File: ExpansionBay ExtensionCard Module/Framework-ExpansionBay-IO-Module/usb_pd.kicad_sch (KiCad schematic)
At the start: 9 parts, among them U2 CYPD4126-40LQXIT

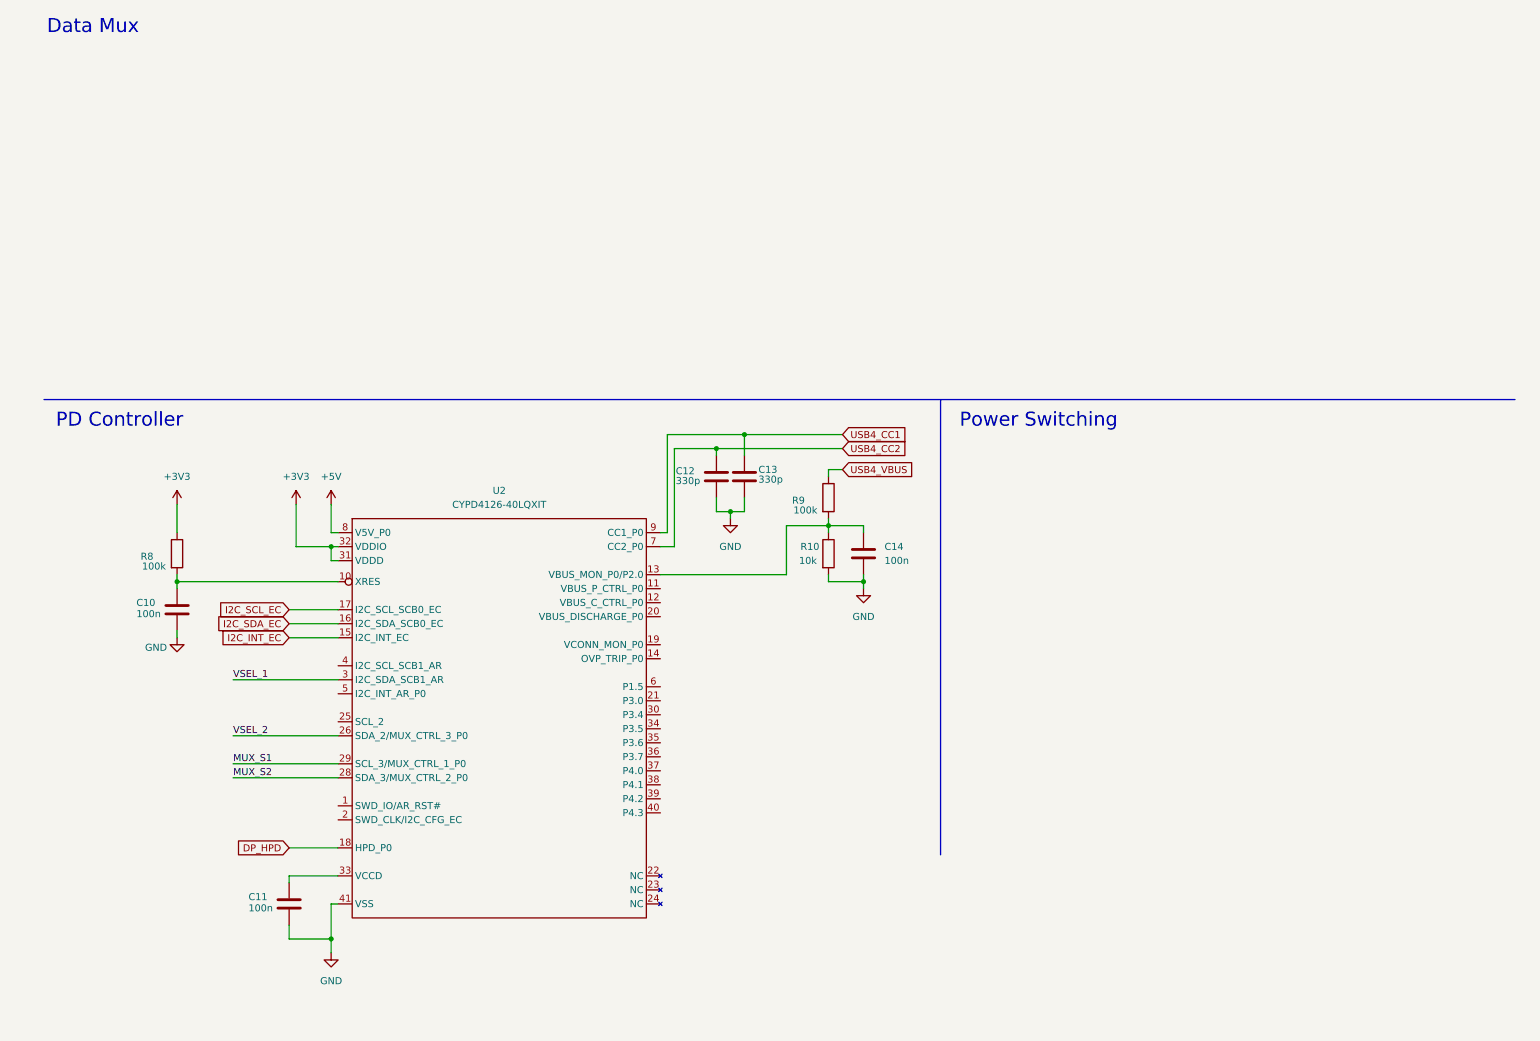
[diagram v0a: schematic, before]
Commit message: partial redesign
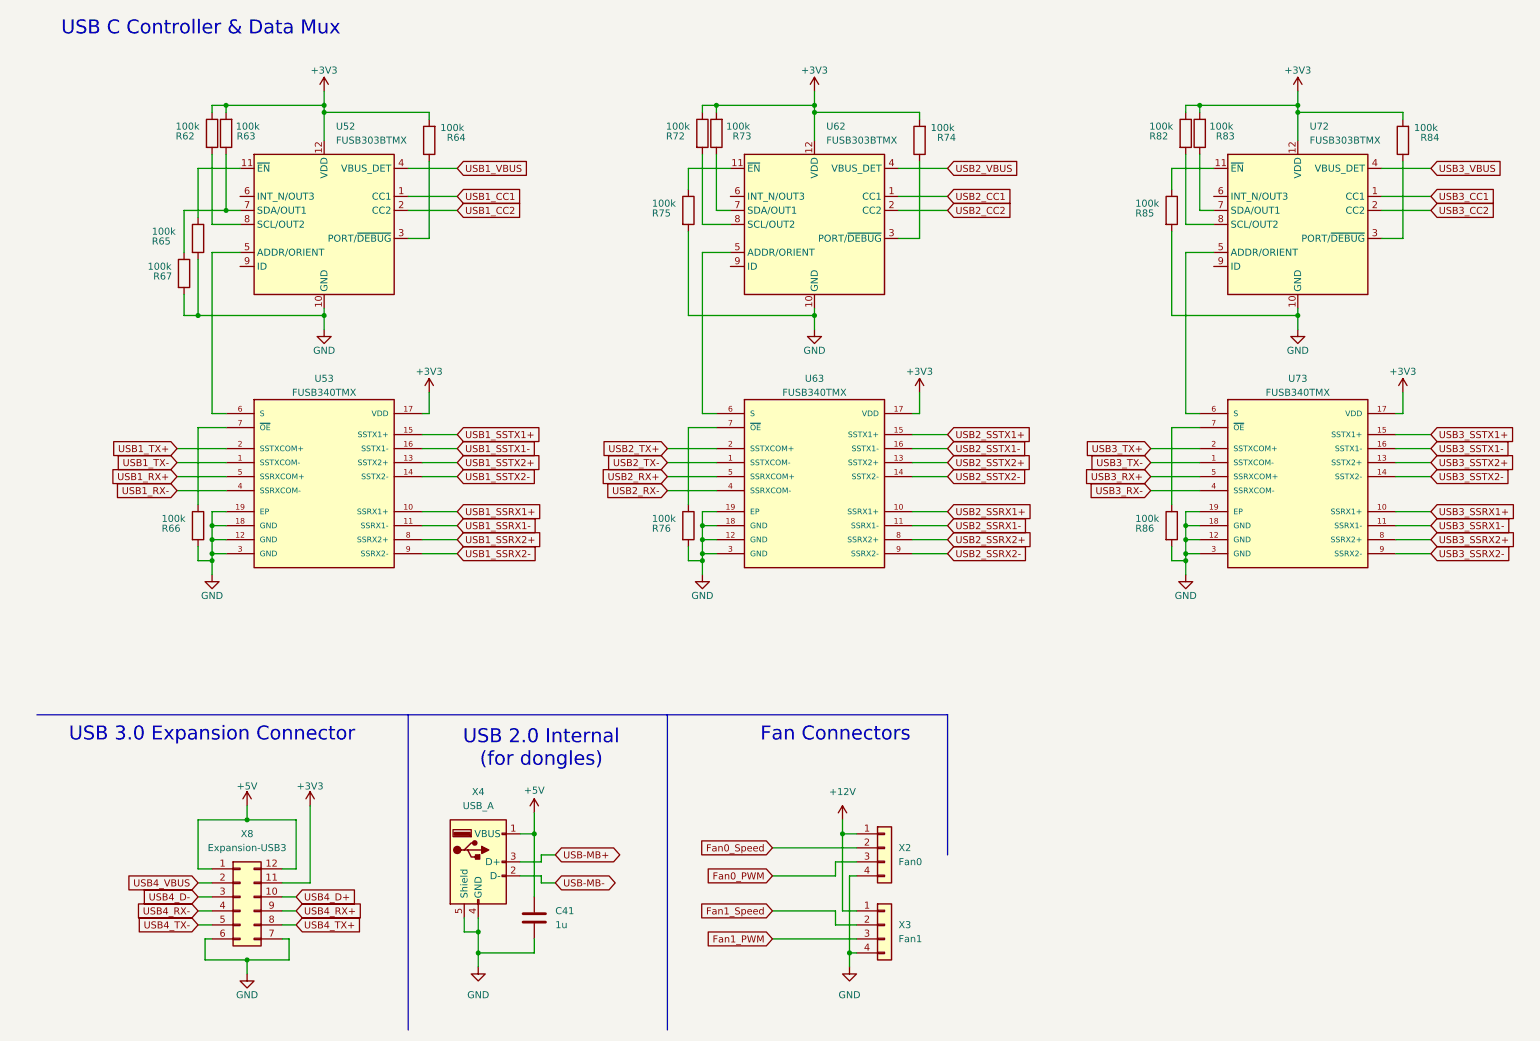
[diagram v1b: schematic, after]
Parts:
- removed C10, C11, C14: 100n, symbol Device:C
- removed C12, C13: 330p, symbol Device:C
- removed R10: 10k, symbol Device:R
- removed R8, R9: 100k, symbol Device:R
- removed U2: CYPD4126-40LQXIT, Package_DFN_QFN:QFN-40-1EP_6x6mm_P0.5mm_EP4.6x4.6mm, symbol Framework-ExpansionBay-IOModule:CYPD4126-40LQXIT
- added C41: 1u, symbol Device:C
- added R62, R63, R64, R65, R66, R67, R72, R73, R74, R75, R76, R82, R83, R84, R85, R86: 100k, Resistor_SMD:R_0805_2012Metric, symbol Device:R
- added U52, U62, U72: FUSB303BTMX, Package_DFN_QFN:Texas_X2QFN-12_1.6x1.6mm_P0.4mm, symbol Interface_USB:FUSB303BTMX
- added U53, U63, U73: FUSB340TMX, Framework-ExpansionBay-IOModule:QFN40P200X280X40-19N, symbol Framework-ExpansionBay-IOModule:FUSB340TMX
- added X2: Fan0, Framework-ExpansionBay:Molex-52746-0471, symbol Connector_Generic:Conn_01x04
- added X3: Fan1, Framework-ExpansionBay:Molex-52746-0471, symbol Connector_Generic:Conn_01x04
- added X4: USB_A, Framework-ExpansionBay-IOModule:Würth-USB2-629104190121, symbol Connector:USB_A
- added X8: Expansion-USB3, Framework-ExpansionBay-IOModule:DS1015-02-12R6, symbol Connector_Generic:Conn_02x06_Counter_Clockwise
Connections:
- net +3V3: now also R62.1, R63.2, R64.2, R72.1, R73.2, R74.2, R82.1, R83.2, R84.2, U52.12 (VDD), U53.17 (VDD), U62.12 (VDD), U63.17 (VDD), U72.12 (VDD), U73.17 (VDD), X8.11 (Pin_11)
- net +5V: now also C41.1, X4.1 (VBUS), X8.1 (Pin_1), X8.12 (Pin_12)
- net GND: now also C41.2, R65.2, R66.2, R67.2, R75.2, R76.2, R85.2, R86.2, U52.10 (GND), U53.12 (GND), U53.18 (GND), U53.19 (EP), U53.3 (GND), U62.10 (GND), U63.12 (GND), U63.18 (GND), U63.19 (EP), U63.3 (GND), U72.10 (GND), U73.12 (GND), U73.18 (GND), U73.19 (EP), U73.3 (GND), X2.4 (Pin_4), X3.4 (Pin_4), X4.4 (GND), X4.5 (Shield), X8.6 (Pin_6), X8.7 (Pin_7)
- net USB4_VBUS: now also X8.2 (Pin_2)
- new net: R64.1, U52.3 (PORT/~{DEBUG})
- new net: U72.5 (ADDR/ORIENT), U73.6 (S)
- new net: R86.1, U73.7 (~{OE})
- new net: R72.2, U62.8 (SCL/OUT2)
- new net: R62.2, U52.8 (SCL/OUT2)
- new net: R73.1, U62.7 (SDA/OUT1)
- new net: R75.1, U62.11 (~{EN})
- new net: R74.1, U62.3 (PORT/~{DEBUG})
- new net: U62.5 (ADDR/ORIENT), U63.6 (S)
- new net: R83.1, U72.7 (SDA/OUT1)
- new net: R76.1, U63.7 (~{OE})
- new net: R65.1, U52.11 (~{EN})
- new net: U52.5 (ADDR/ORIENT), U53.6 (S)
- new net: R63.1, R67.1, U52.7 (SDA/OUT1)
- new net: R66.1, U53.7 (~{OE})
- new net: R84.1, U72.3 (PORT/~{DEBUG})
- new net: R85.1, U72.11 (~{EN})
- new net: R82.2, U72.8 (SCL/OUT2)
- new net +12V: X2.1 (Pin_1), X3.1 (Pin_1)
- new net Fan0_PWM: X2.3 (Pin_3)
- new net Fan0_Speed: X2.2 (Pin_2)
- new net Fan1_PWM: X3.3 (Pin_3)
- new net Fan1_Speed: X3.2 (Pin_2)
- new net USB-MB+: X4.3 (D+)
- new net USB-MB-: X4.2 (D-)
- new net USB1_CC1: U52.1 (CC1)
- new net USB1_CC2: U52.2 (CC2)
- new net USB1_RX+: U53.5 (SSRXCOM+)
- new net USB1_RX-: U53.4 (SSRXCOM-)
- new net USB1_SSRX1+: U53.10 (SSRX1+)
- new net USB1_SSRX1-: U53.11 (SSRX1-)
- new net USB1_SSRX2+: U53.8 (SSRX2+)
- new net USB1_SSRX2-: U53.9 (SSRX2-)
- new net USB1_SSTX1+: U53.15 (SSTX1+)
- new net USB1_SSTX1-: U53.16 (SSTX1-)
- new net USB1_SSTX2+: U53.13 (SSTX2+)
- new net USB1_SSTX2-: U53.14 (SSTX2-)
- new net USB1_TX+: U53.2 (SSTXCOM+)
- new net USB1_TX-: U53.1 (SSTXCOM-)
- new net USB1_VBUS: U52.4 (VBUS_DET)
- new net USB2_CC1: U62.1 (CC1)
- new net USB2_CC2: U62.2 (CC2)
- new net USB2_RX+: U63.5 (SSRXCOM+)
- new net USB2_RX-: U63.4 (SSRXCOM-)
- new net USB2_SSRX1+: U63.10 (SSRX1+)
- new net USB2_SSRX1-: U63.11 (SSRX1-)
- new net USB2_SSRX2+: U63.8 (SSRX2+)
- new net USB2_SSRX2-: U63.9 (SSRX2-)
- new net USB2_SSTX1+: U63.15 (SSTX1+)
- new net USB2_SSTX1-: U63.16 (SSTX1-)
- new net USB2_SSTX2+: U63.13 (SSTX2+)
- new net USB2_SSTX2-: U63.14 (SSTX2-)
- new net USB2_TX+: U63.2 (SSTXCOM+)
- new net USB2_TX-: U63.1 (SSTXCOM-)
- new net USB2_VBUS: U62.4 (VBUS_DET)
- new net USB3_CC1: U72.1 (CC1)
- new net USB3_CC2: U72.2 (CC2)
- new net USB3_RX+: U73.5 (SSRXCOM+)
- new net USB3_RX-: U73.4 (SSRXCOM-)
- new net USB3_SSRX1+: U73.10 (SSRX1+)
- new net USB3_SSRX1-: U73.11 (SSRX1-)
- new net USB3_SSRX2+: U73.8 (SSRX2+)
- new net USB3_SSRX2-: U73.9 (SSRX2-)
- new net USB3_SSTX1+: U73.15 (SSTX1+)
- new net USB3_SSTX1-: U73.16 (SSTX1-)
- new net USB3_SSTX2+: U73.13 (SSTX2+)
- new net USB3_SSTX2-: U73.14 (SSTX2-)
- new net USB3_TX+: U73.2 (SSTXCOM+)
- new net USB3_TX-: U73.1 (SSTXCOM-)
- new net USB3_VBUS: U72.4 (VBUS_DET)
- new net USB4_D+: X8.10 (Pin_10)
- new net USB4_D-: X8.3 (Pin_3)
- new net USB4_RX+: X8.9 (Pin_9)
- new net USB4_RX-: X8.4 (Pin_4)
- new net USB4_TX+: X8.8 (Pin_8)
- new net USB4_TX-: X8.5 (Pin_5)
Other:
- note added: "Fan Connectors"
- note added: "USB 2.0 Internal (for dongles)"
- note added: "USB 3.0 Expansion Connector"
- note added: "USB C Controller & Data Mux"
- note removed: "Data Mux"
- note removed: "PD Controller"
- note removed: "Power Switching"
